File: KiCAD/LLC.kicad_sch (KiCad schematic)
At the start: 1 part, among them U1 UCC25661-Q1

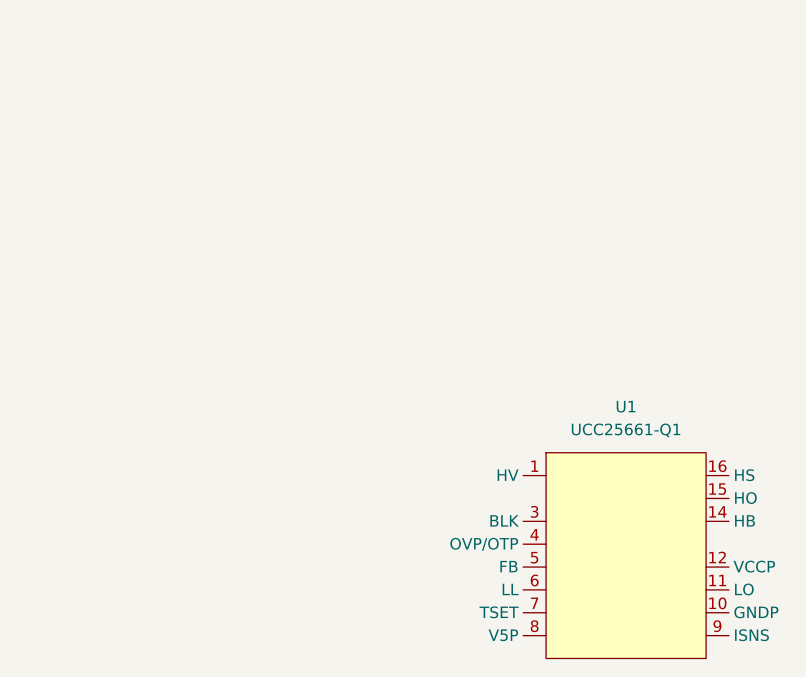
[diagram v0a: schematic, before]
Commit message: kicad stuff
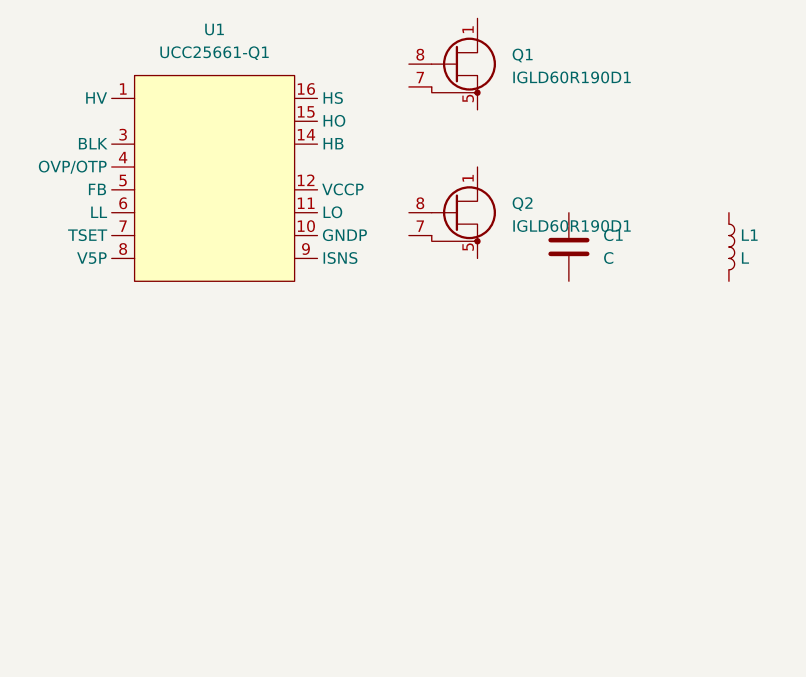
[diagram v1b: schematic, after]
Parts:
- added C1: C, symbol Device:C
- added L1: L, symbol Device:L
- added Q1, Q2: IGLD60R190D1, Package_SON:Infineon_PG-LSON-8-1, symbol Transistor_FET:IGLD60R190D1
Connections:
- new net: Q1.1 (D), Q1.2 (D), Q1.3 (D), Q1.4 (D)
- new net: Q1.5 (S), Q1.6 (S), Q1.9 (S)
- new net: Q2.1 (D), Q2.2 (D), Q2.3 (D), Q2.4 (D)
- new net: Q2.5 (S), Q2.6 (S), Q2.9 (S)
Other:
- moved on the sheet: U1
